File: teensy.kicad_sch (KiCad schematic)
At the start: 6 parts

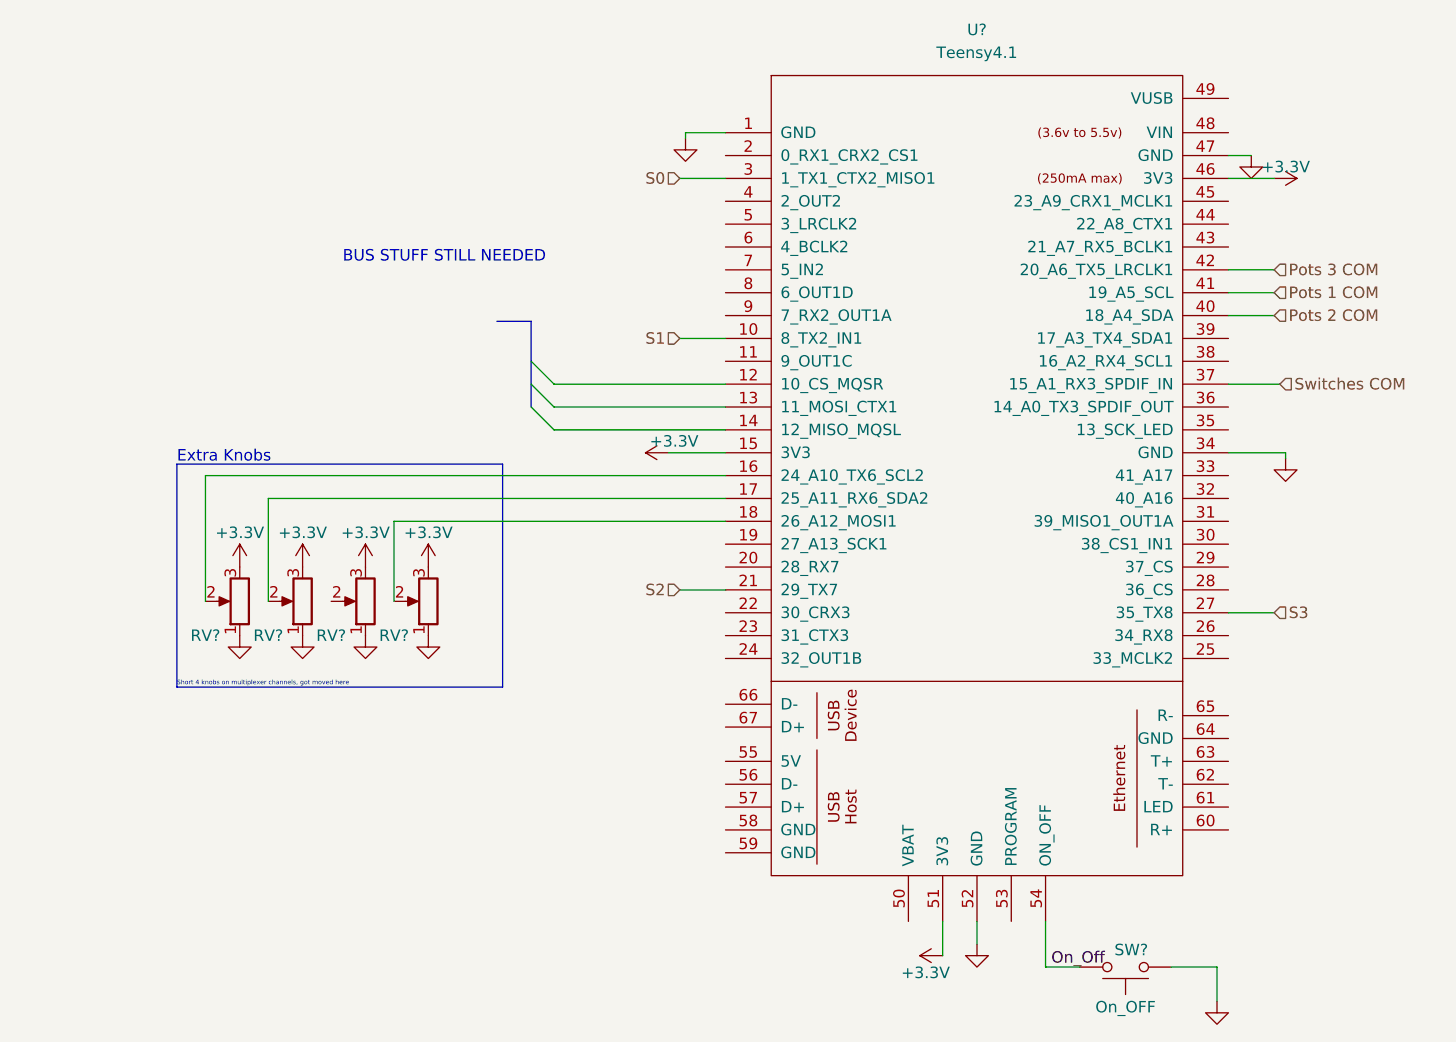
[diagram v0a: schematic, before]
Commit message: First Round ERC Checks
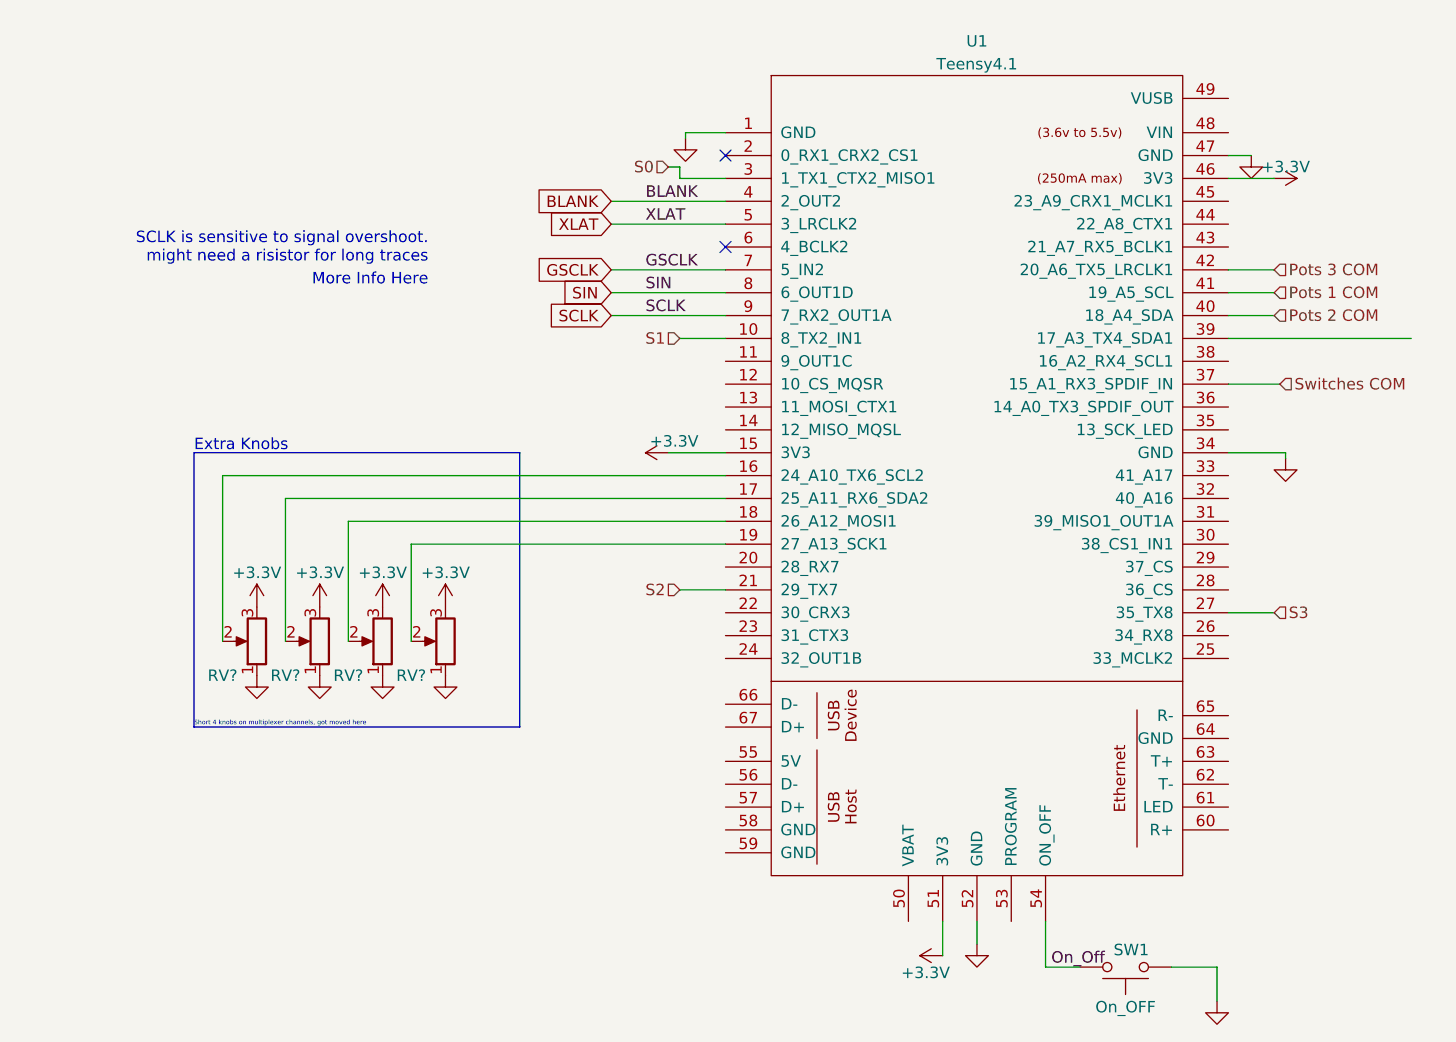
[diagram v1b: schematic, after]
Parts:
- gave numbers to parts that had none: 2
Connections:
- net at RV?.2: now also U1.19 (27_A13_SCK1); no longer U1.18 (26_A12_MOSI1)
- net BLANK: now reaches U1.4 (2_OUT2)
- net XLAT: now reaches U1.5 (3_LRCLK2)
- net GSCLK: now reaches U1.7 (5_IN2)
- net SIN: now reaches U1.8 (6_OUT1D)
- net SCLK: now reaches U1.9 (7_RX2_OUT1A)
- net at RV?.2: now also U1.18 (26_A12_MOSI1)
- no-connect marks 0 -> 2
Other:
- note added: "More Info Here"
- note added: "SCLK is sensitive to signal overshoot. might need a risistor for long traces"
- note removed: "BUS STUFF STILL NEEDED"
- moved on the sheet: RV?
